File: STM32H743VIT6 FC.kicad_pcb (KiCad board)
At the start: 4 copper layers, 37 x 37 mm, 93 parts, among them J1 USB4730-GF-A, SW2 Y78B22310FP, U1 TPS54302DDCR, U2 USBLC6-2SC6, U3 TPS54302DDCR

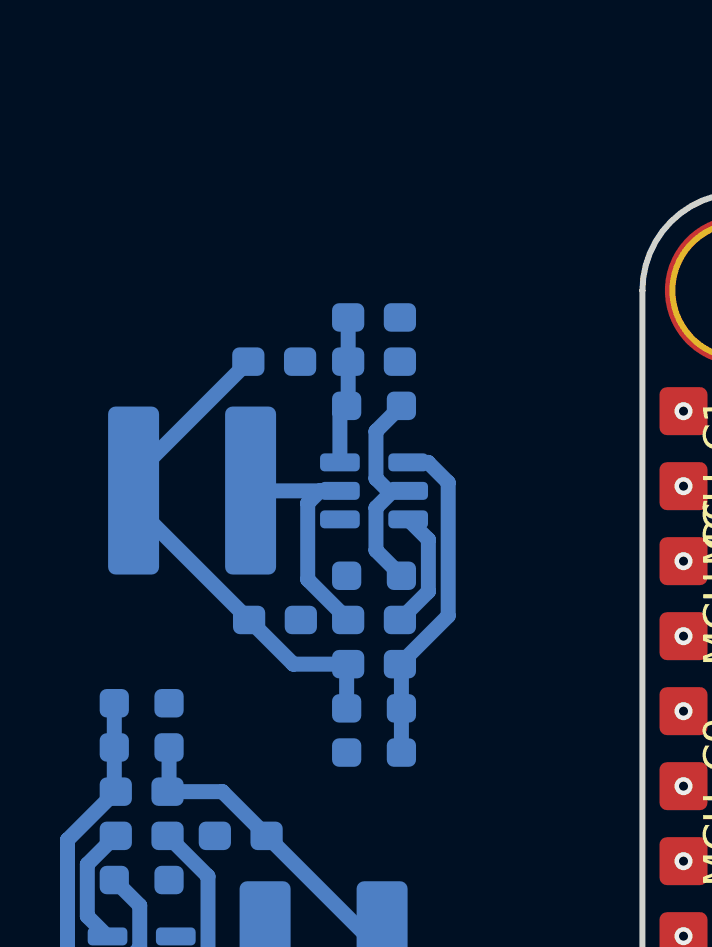
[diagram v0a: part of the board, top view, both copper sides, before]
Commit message: min
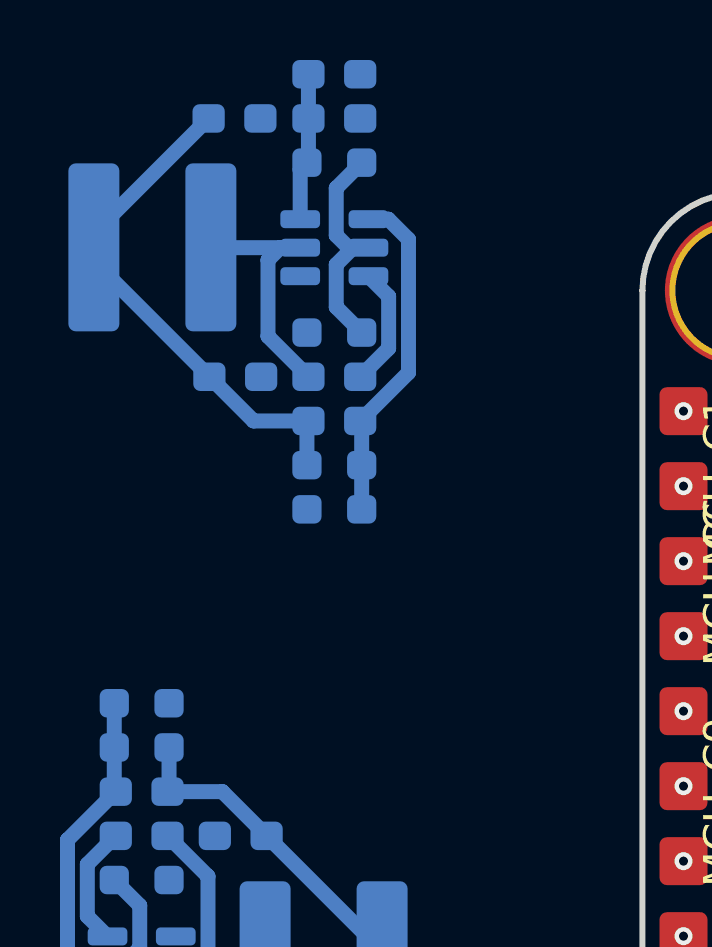
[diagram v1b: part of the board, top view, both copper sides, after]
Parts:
- moved 9V_C11 8.21 mm to (133.7, 99.3)
- moved 9V_C12 8.21 mm to (137.0, 109.3)
- moved 9V_C8 8.21 mm to (137.0, 99.3)
- moved 9V_C9 8.21 mm to (137.0, 107.9)
- moved 9V_R5 8.21 mm to (137.0, 100.7)
- moved 9V_R6 8.21 mm to (137.0, 106.4)
- moved 9V_R7 8.21 mm to (137.0, 110.8)
- moved 9V_R8 8.21 mm to (137.0, 112.3)
- moved U3 8.21 mm to (137.0, 103.6)
- moved 9V_C10 8.21 mm to (133.7, 107.9)
- moved 9V_L1 8.21 mm to (130.9, 103.6)
- moved 9V_C7 8.21 mm to (137.0, 97.8)

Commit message: Removed EN resistors from bucks.
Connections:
- U1 pad 5: Net-(U1-EN) -> unconnected-(U1-EN-Pad5)
- U3 pad 5: Net-(U3-EN) -> unconnected-(U3-EN-Pad5)
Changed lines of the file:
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@@
 	(net 127 "unconnected-(J1-DN1-PadA7)")
 	(net 128 "3.3VA")
+	(net 129 "unconnected-(U1-EN-Pad5)")
+	(net 130 "unconnected-(U3-EN-Pad5)")
 	(footprint "Resistor_SMD:R_0603_1608Metric_Pad0.98x0.95mm_HandSolder"
 		(layer "F.Cu")
@@
 			(layers "B.Cu" "B.Mask" "B.Paste")
 			(roundrect_rratio 0.25)
-			(net 20 "Net-(U3-EN)")
+			(net 130 "unconnected-(U3-EN-Pad5)")
 			(pinfunction "EN")
-			(pintype "input")
+			(pintype "input+no_connect")
 		)
 		(pad "6" smd roundrect
@@
 			(layers "B.Cu" "B.Mask" "B.Paste")
 			(roundrect_rratio 0.25)
-			(net 14 "Net-(U1-EN)")
+			(net 129 "unconnected-(U1-EN-Pad5)")
 			(pinfunction "EN")
-			(pintype "input")
+			(pintype "input+no_connect")
 		)
 		(pad "6" smd roundrect
